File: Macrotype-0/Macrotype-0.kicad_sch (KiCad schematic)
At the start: 30 parts, among them U1 ProMicro

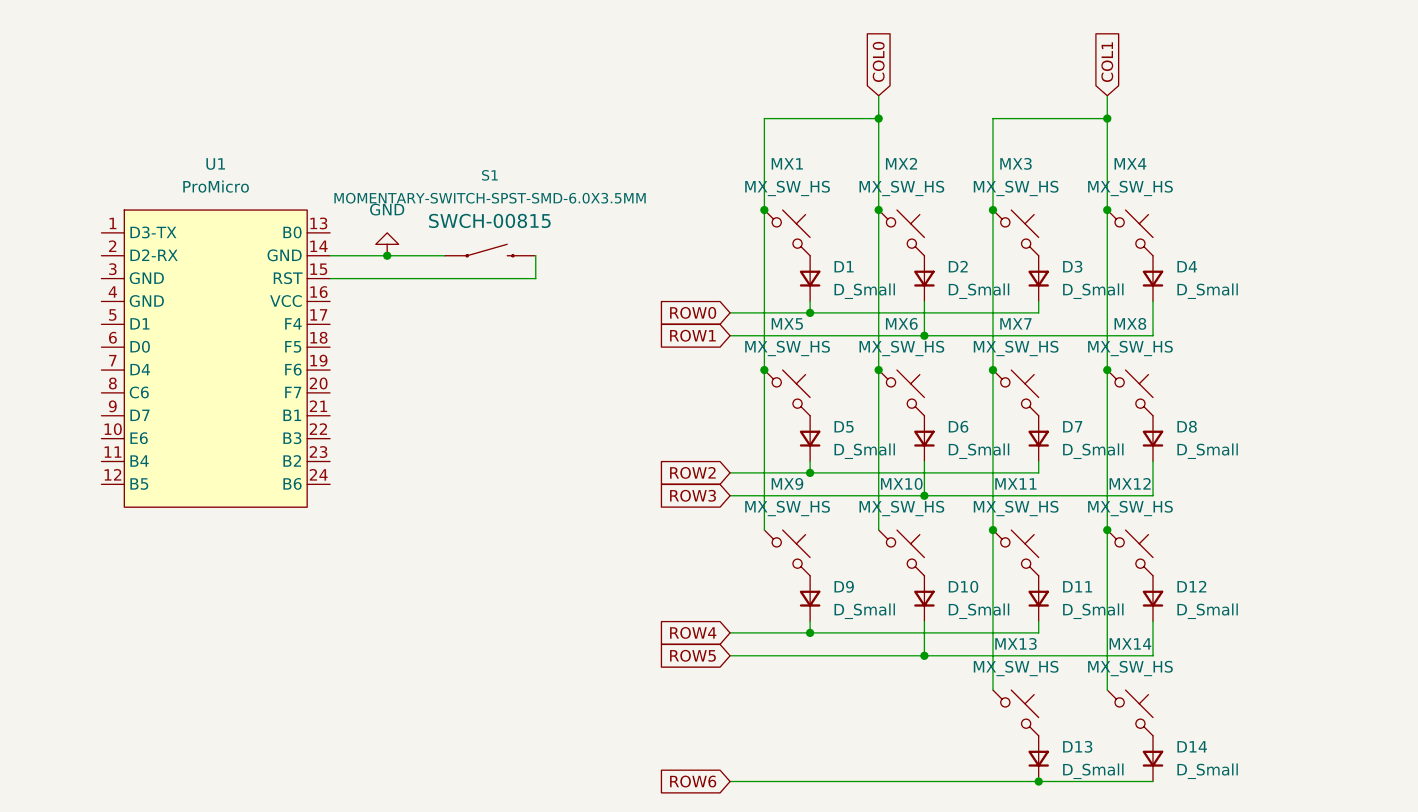
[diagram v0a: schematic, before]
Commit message: Update 1.0
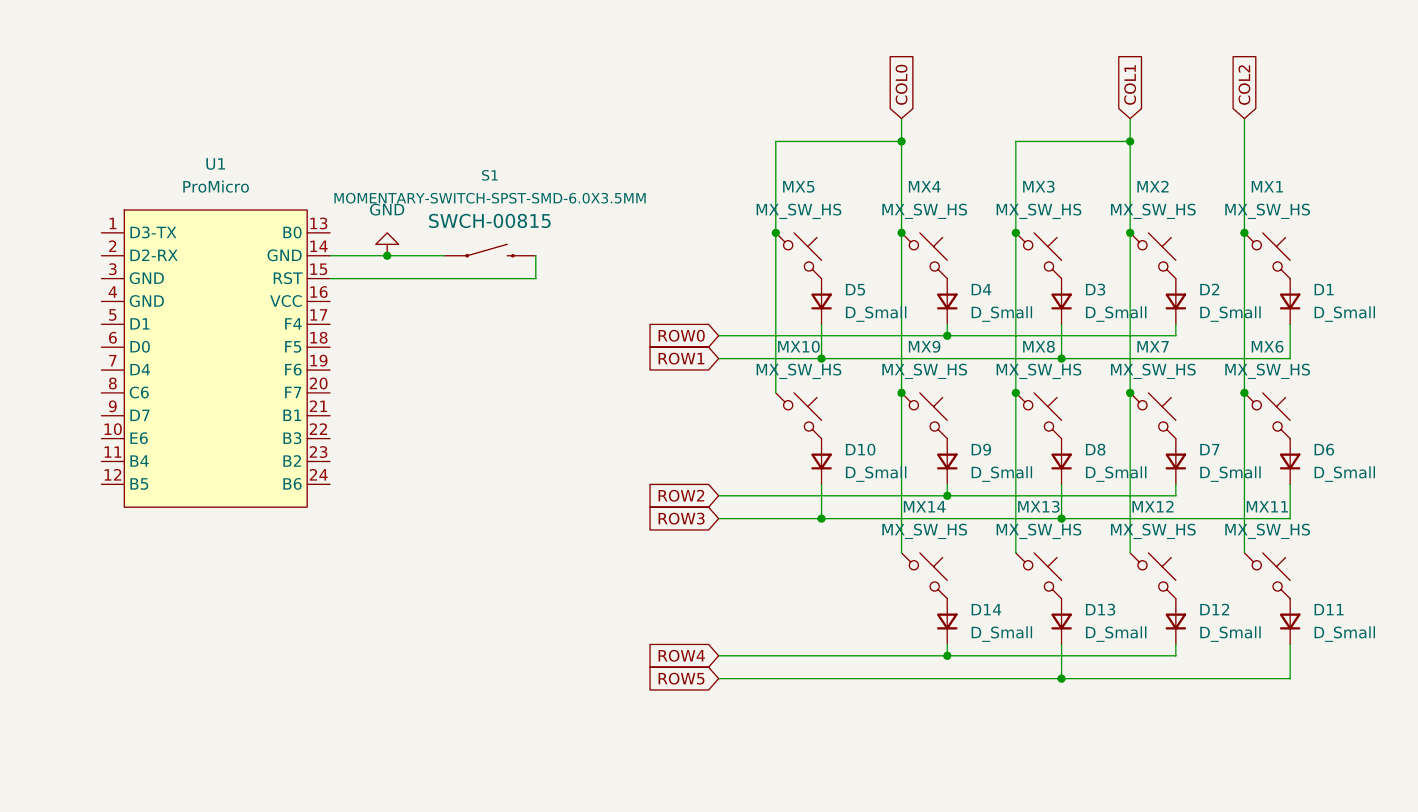
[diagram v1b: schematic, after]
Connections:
- net COL0: now also MX14.1, MX4.1; no longer MX1.1, MX2.1, MX6.1
- net COL1: now also MX2.1; no longer MX11.1, MX14.1, MX4.1
- net ROW0: now also D2.1 (K), D4.1 (K); no longer D1.1 (K), D3.1 (K)
- net ROW1: now also D1.1 (K), D3.1 (K), D5.1 (K); no longer D2.1 (K), D4.1 (K)
- net ROW2: now also D9.1 (K); no longer D5.1 (K)
- net ROW3: now also D10.1 (K)
- net ROW4: now also D12.1 (K), D14.1 (K); no longer D11.1 (K), D9.1 (K)
- net ROW5: now also D11.1 (K), D13.1 (K); no longer D10.1 (K), D12.1 (K)
- removed net ROW6: D13.1 (K), D14.1 (K)
- new net COL2: MX1.1, MX11.1, MX6.1
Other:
- moved on the sheet: D1, D10, D11, D12, D13, D14, D2, D3, D4, D5, D6, D7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

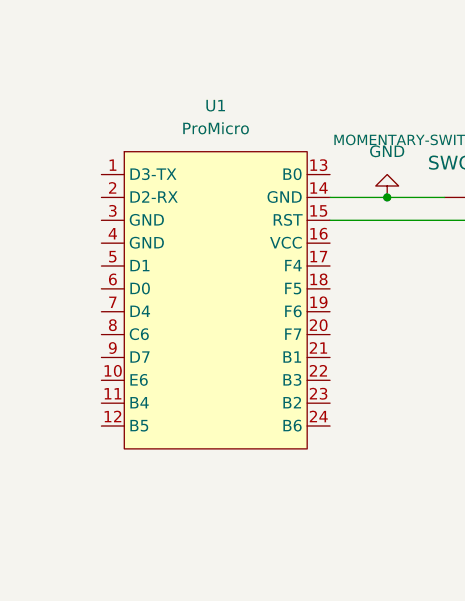
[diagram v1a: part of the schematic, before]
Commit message: Update 1.2
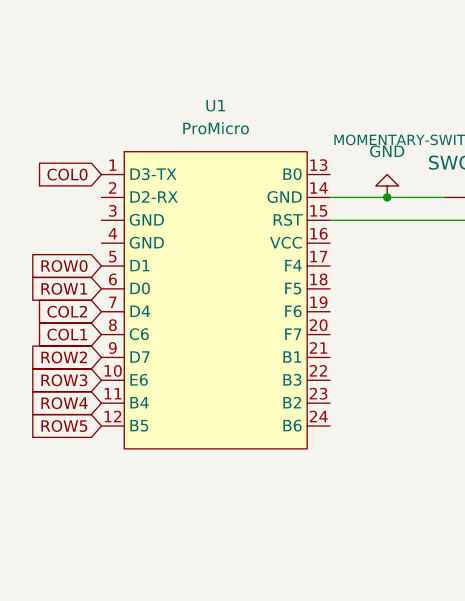
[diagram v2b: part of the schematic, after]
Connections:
- net COL0: now also U1.1 (D3-TX)
- net COL1: now also U1.8 (C6)
- net COL2: now also U1.7 (D4)
- net ROW0: now also U1.5 (D1)
- net ROW1: now also U1.6 (D0)
- net ROW2: now also U1.9 (D7)
- net ROW3: now also U1.10 (E6)
- net ROW4: now also U1.11 (B4)
- net ROW5: now also U1.12 (B5)
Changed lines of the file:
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@@
+    )
+  )
+  (global_label "ROW4" (shape input) (at 50.8 88.9 180) (fields_autoplaced)
+    (effects (font (size 1.27 1.27)) (justify right))
+    (property "Intersheetrefs" "${INTERSHEET_REFS}" (at 42.6328 88.9 0)
+      (effects (font (size 1.27 1.27)) (justify right) hide)
+    )
+  )
+  (global_label "ROW5" (shape input) (at 50.8 91.44 180) (fields_autoplaced)
+    (effects (font (size 1.27 1.27)) (justify right))
+    (property "Intersheetrefs" "${INTERSHEET_REFS}" (at 42.6328 91.44 0)
+      (effects (font (size 1.27 1.27)) (justify right) hide)
     )
   )
@@
     )
   )
+  (global_label "COL1" (shape input) (at 50.8 81.28 180) (fields_autoplaced)
+    (effects (font (size 1.27 1.27)) (justify right))
+    (property "Intersheetrefs" "${INTERSHEET_REFS}" (at 43.0561 81.28 0)
+      (effects (font (size 1.27 1.27)) (justify right) hide)
+    )
+  )
   (global_label "COL2" (shape input) (at 177.8 50.8 90) (fields_autoplaced)
     (effects (font (size 1.27 1.27)) (justify left))
     (property "Intersheetrefs" "${INTERSHEET_REFS}" (at 177.8 43.0561 90)
       (effects (font (size 1.27 1.27)) (justify left) hide)
+    )
+  )
+  (global_label "COL0" (shape input) (at 50.8 63.5 180) (fields_autoplaced)
+    (effects (font (size 1.27 1.27)) (justify right))
+    (property "Intersheetrefs" "${INTERSHEET_REFS}" (at 43.0561 63.5 0)
+      (effects (font (size 1.27 1.27)) (justify right) hide)
+    )
+  )
+  (global_label "ROW2" (shape input) (at 50.8 83.82 180) (fields_autoplaced)
+    (effects (font (size 1.27 1.27)) (justify right))
+    (property "Intersheetrefs" "${INTERSHEET_REFS}" (at 42.6328 83.82 0)
+      (effects (font (size 1.27 1.27)) (justify right) hide)
+    )
+  )
+  (global_label "ROW1" (shape input) (at 50.8 76.2 180) (fields_autoplaced)
+    (effects (font (size 1.27 1.27)) (justify right))
+    (property "Intersheetrefs" "${INTERSHEET_REFS}" (at 42.6328 76.2 0)
+      (effects (font (size 1.27 1.27)) (justify right) hide)
     )
   )
@@
     )
   )
+  (global_label "ROW0" (shape input) (at 50.8 73.66 180) (fields_autoplaced)
+    (effects (font (size 1.27 1.27)) (justify right))
+    (property "Intersheetrefs" "${INTERSHEET_REFS}" (at 42.6328 73.66 0)
+      (effects (font (size 1.27 1.27)) (justify right) hide)
+    )
+  )
   (global_label "ROW5" (shape input) (at 119.38 113.03 180) (fields_autoplaced)
     (effects (font (size 1.27 1.27)) (justify right))
@@
       (effects (font (size 1.27 1.27)) (justify right) hide)
     )
+  )
+  (global_label "ROW3" (shape input) (at 50.8 86.36 180) (fields_autoplaced)
+    (effects (font (size 1.27 1.27)) (justify right))
+    (property "Intersheetrefs" "${INTERSHEET_REFS}" (at 42.6328 86.36 0)
+      (effects (font (size 1.27 1.27)) (justify right) hide)
+    )
+  )
+  (global_label "COL2" (shape input) (at 50.8 78.74 180) (fields_autoplaced)
+    (effects (font (size 1.27 1.27)) (justify right))
+    (property "Intersheetrefs" "${INTERSHEET_REFS}" (at 43.0561 78.74 0)
+      (effects (font (size 1.27 1.27)) (justify right) hide)
+    )
